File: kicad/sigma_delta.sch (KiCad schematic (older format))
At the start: 34 parts, among them U1801 SI8661BD, U1802 SI8661BD, U1803 SN74LVC2G17DBVR, U1804 SN74LVC2G17DBVR

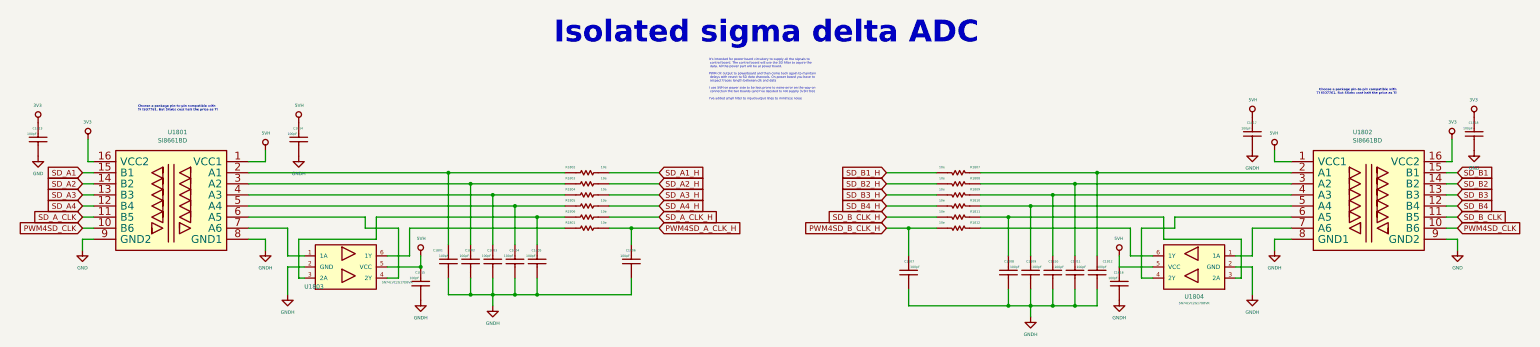
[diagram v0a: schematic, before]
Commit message: beginine routing... far far away
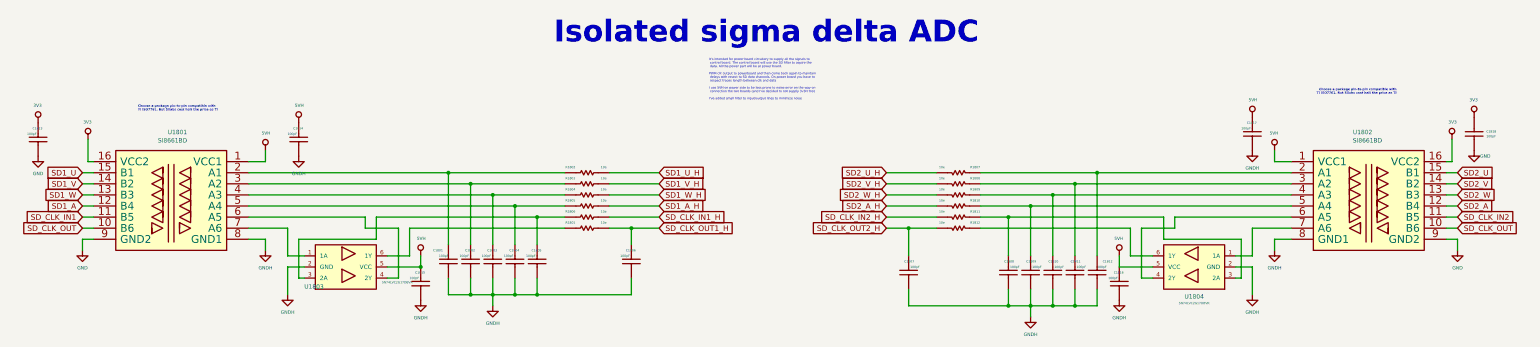
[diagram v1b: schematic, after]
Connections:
- net PWM4SD_A_CLK_H renamed SD_CLK_OUT1_H
- net PWM4SD_B_CLK_H renamed SD_CLK_OUT2_H
- net PWM4SD_CLK renamed SD_CLK_OUT
- net SD_A1 renamed SD1_U
- net SD_A1_H renamed SD1_U_H
- net SD_A2 renamed SD1_V
- net SD_A2_H renamed SD1_V_H
- net SD_A3 renamed SD1_W
- net SD_A3_H renamed SD1_W_H
- net SD_A4 renamed SD1_A
- net SD_A4_H renamed SD1_A_H
- net SD_A_CLK renamed SD_CLK_IN1
- net SD_A_CLK_H renamed SD_CLK_IN1_H
- net SD_B1 renamed SD2_U
- net SD_B1_H renamed SD2_U_H
- net SD_B2 renamed SD2_V
- net SD_B2_H renamed SD2_V_H
- net SD_B3 renamed SD2_W
- net SD_B3_H renamed SD2_W_H
- net SD_B4 renamed SD2_A
- net SD_B4_H renamed SD2_A_H
- net SD_B_CLK renamed SD_CLK_IN2
- net SD_B_CLK_H renamed SD_CLK_IN2_H
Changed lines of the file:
@@
 Isolated sigma delta ADC
 Text GLabel 2700 3350 0    50   Input ~ 0
-SD_A_CLK
+SD_CLK_IN1
 $Comp
 L servo:GND #PWR?
@@
 	-1   0    0    -1
 $EndComp
-Text GLabel 2700 3450 0    50   Input ~ 0
-PWM4SD_CLK
 $Comp
 L servo:3V3 #PWR?
@@
 	2750 2650 2750 2850
 Text GLabel 2700 2950 0    50   Input ~ 0
-SD_A1
+SD1_U
 Text GLabel 2700 3050 0    50   Input ~ 0
-SD_A2
+SD1_V
 Text GLabel 2700 3150 0    50   Input ~ 0
-SD_A3
+SD1_W
 Text GLabel 2700 3250 0    50   Input ~ 0
-SD_A4
+SD1_A
 $Comp
 L servo:GNDH #PWR?
@@
 Wire Wire Line
 	7450 3350 7900 3350
-Text GLabel 15100 3350 2    50   Input ~ 0
-SD_B_CLK
 $Comp
 L servo:GND #PWR?
@@
 	1    0    0    -1
 $EndComp
-Text GLabel 15100 3450 2    50   Input ~ 0
-PWM4SD_CLK
 $Comp
 L servo:3V3 #PWR?
@@
 Wire Wire Line
 	15050 2650 15050 2850
-Text GLabel 15100 2950 2    50   Input ~ 0
-SD_B1
-Text GLabel 15100 3050 2    50   Input ~ 0
-SD_B2
-Text GLabel 15100 3150 2    50   Input ~ 0
-SD_B3
-Text GLabel 15100 3250 2    50   Input ~ 0
-SD_B4
 $Comp
 L servo:GNDH #PWR?
@@
 Wire Wire Line
 	11250 4250 11250 4150
-Text GLabel 7900 2950 2    50   Input ~ 0
-SD_A1_H
-Text GLabel 7900 3050 2    50   Input ~ 0
-SD_A2_H
-Text GLabel 7900 3150 2    50   Input ~ 0
-SD_A3_H
-Text GLabel 7900 3250 2    50   Input ~ 0
-SD_A4_H
-Text GLabel 7900 3350 2    50   Input ~ 0
-SD_A_CLK_H
-Text GLabel 7900 3450 2    50   Input ~ 0
-PWM4SD_A_CLK_H
-Text GLabel 9950 2950 0    50   Input ~ 0
-SD_B1_H
-Text GLabel 9950 3050 0    50   Input ~ 0
-SD_B2_H
-Text GLabel 9950 3150 0    50   Input ~ 0
-SD_B3_H
-Text GLabel 9950 3250 0    50   Input ~ 0
-SD_B4_H
-Text GLabel 9950 3350 0    50   Input ~ 0
-SD_B_CLK_H
-Text GLabel 9950 3450 0    50   Input ~ 0
-PWM4SD_B_CLK_H
 $Comp
 L servo:SN74LVC2G17DBVR U?
@@
 AR Path="/5EC40F3C/5E3CAD23" Ref="C?"  Part="1"
 AR Path="/6056AA11/5E3CAD23" Ref="C1818"  Part="1"
-F 0 "C1818" V 15400 2700 20  0000 R CNN
-F 1 "100pF" V 15350 2750 20  0000 R CNN
+F 0 "C1818" V 15322 2540 20  0000 R CNN
+F 1 "100pF" V 15279 2540 20  0000 R CNN
 F 2 "servo:C_0603_1608Metric" H 15250 2550 60  0001 C CNN
 F 3 "" H 15250 2650 60  0000 C CNN
@@
 AR Path="/6056AA11/5E3CAD30" Ref="#PWR0245"  Part="1"
 F 0 "#PWR0245" H 15250 2500 30  0001 C CNN
-F 1 "GND" H 15250 2592 30  0000 C CNN
+F 1 "GND" H 15150 2700 30  0000 C CNN
 F 2 "" H 15250 2750 50  0001 C CNN
 F 3 "" H 15250 2750 50  0001 C CNN
@@
 	1    0    0    -1
 $EndComp
+Text GLabel 2700 3450 0    50   Input ~ 0
+SD_CLK_OUT
+Text GLabel 15100 3350 2    50   Input ~ 0
+SD_CLK_IN2
+Text GLabel 15100 2950 2    50   Input ~ 0
+SD2_U
+Text GLabel 15100 3050 2    50   Input ~ 0
+SD2_V
+Text GLabel 15100 3150 2    50   Input ~ 0
+SD2_W
+Text GLabel 15100 3250 2    50   Input ~ 0
+SD2_A
+Text GLabel 15100 3450 2    50   Input ~ 0
+SD_CLK_OUT
+Text GLabel 9950 3350 0    50   Input ~ 0
+SD_CLK_IN2_H
+Text GLabel 9950 2950 0    50   Input ~ 0
+SD2_U_H
+Text GLabel 9950 3050 0    50   Input ~ 0
+SD2_V_H
+Text GLabel 9950 3150 0    50   Input ~ 0
+SD2_W_H
+Text GLabel 9950 3250 0    50   Input ~ 0
+SD2_A_H
+Text GLabel 9950 3450 0    50   Input ~ 0
+SD_CLK_OUT2_H
+Text GLabel 7900 3350 2    50   Input ~ 0
+SD_CLK_IN1_H
+Text GLabel 7900 2950 2    50   Input ~ 0
+SD1_U_H
+Text GLabel 7900 3050 2    50   Input ~ 0
+SD1_V_H
+Text GLabel 7900 3150 2    50   Input ~ 0
+SD1_W_H
+Text GLabel 7900 3250 2    50   Input ~ 0
+SD1_A_H
+Text GLabel 7900 3450 2    50   Input ~ 0
+SD_CLK_OUT1_H
 $EndSCHEMATC
